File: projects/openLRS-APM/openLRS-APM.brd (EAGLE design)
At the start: 43.1 x 20.7 mm, 28 parts, among them IC1 MCP1703CB, IC2 RFM23BPSMD, J1 AVR_SPI_PRG_6PTH, U1 ATMEGA328P, Y1 16MHz

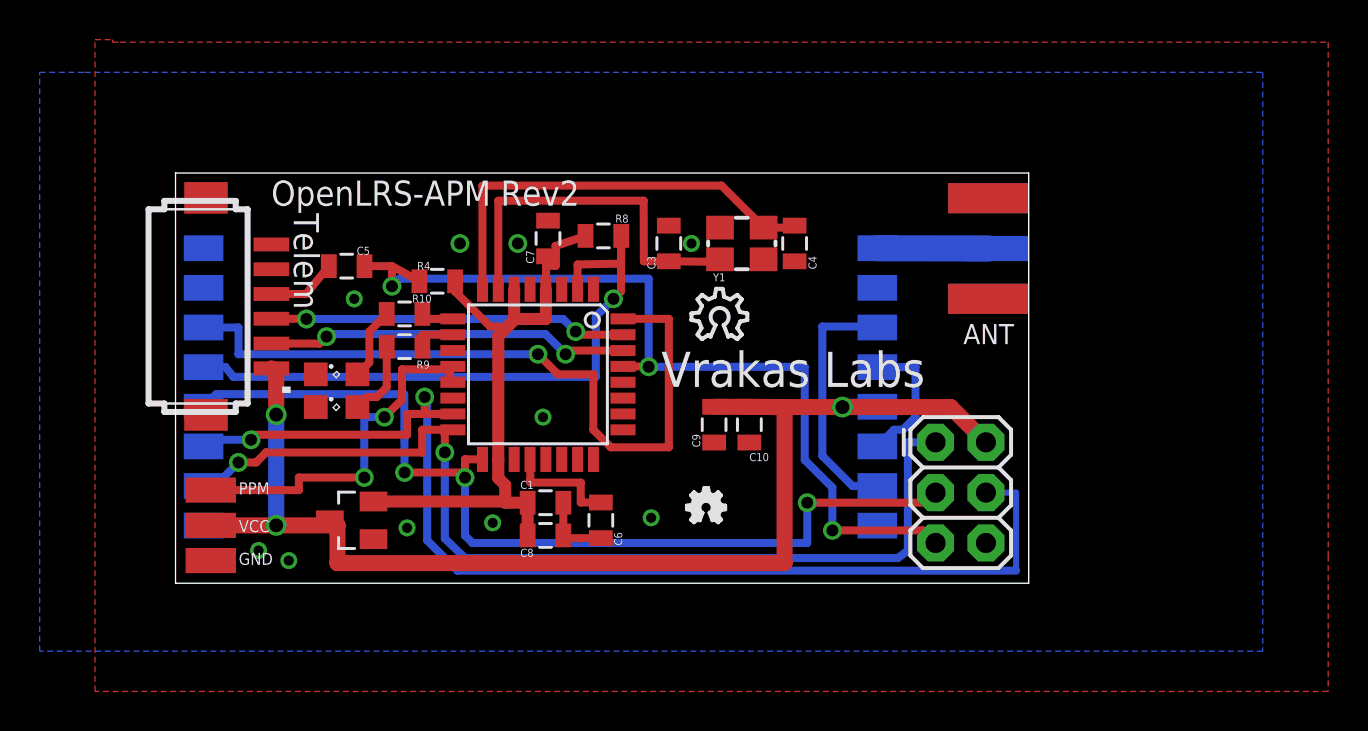
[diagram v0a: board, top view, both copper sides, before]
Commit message: Initial 32u4 USB dongle version
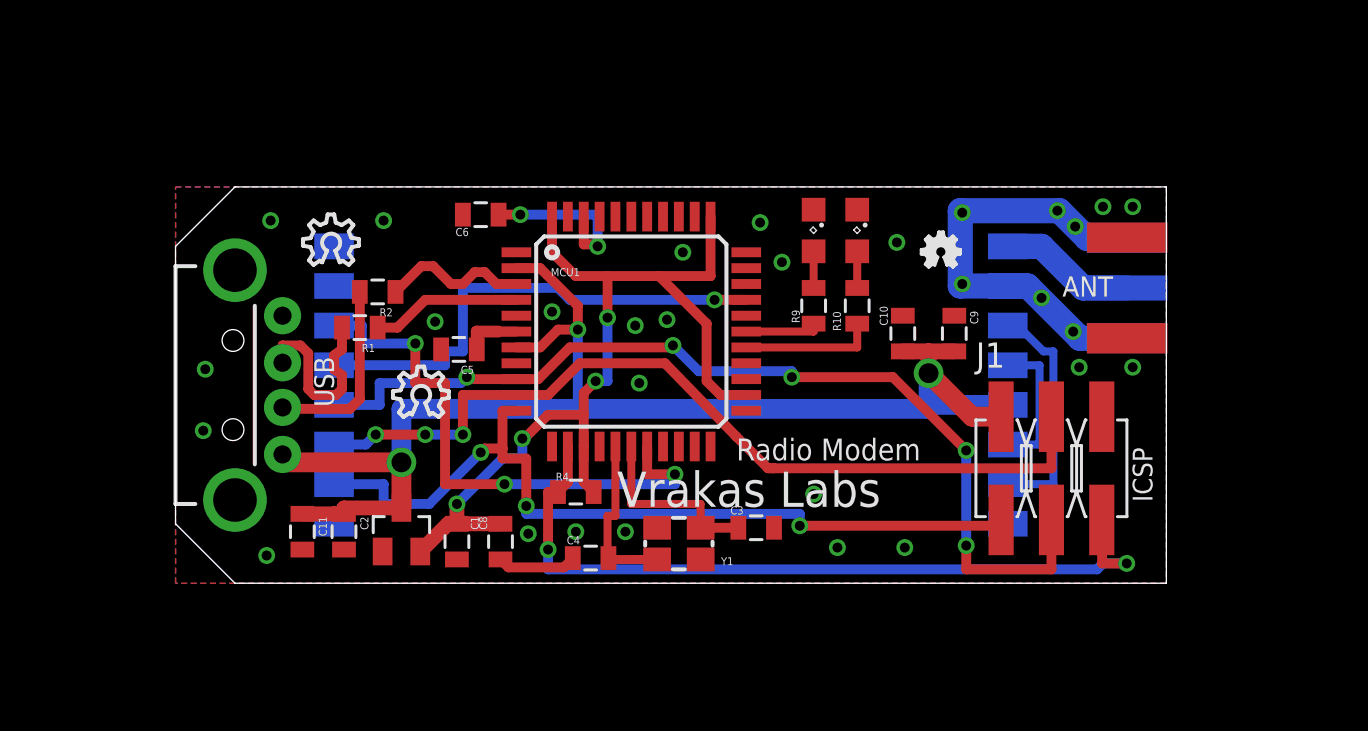
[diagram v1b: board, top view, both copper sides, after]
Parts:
- removed C7: 100n, SparkFun-Capacitors:0805
- removed GND, PPM, VCC: (no value), wirepad:SMD1,27-2,54
- removed R8: 1k, SparkFun-Resistors:0805
- removed TELEMETRY: DF13-6P-1.25H, con-hirose-df13:DF13A-6P-1.25H
- removed U1: ATMEGA328P, SparkFun-DigitalIC:TQFP32-08
- added C11: 100n, SparkFun-Capacitors:0805
- added C2: 1uF, SparkFun-Capacitors:0805
- added JP1: USB-A-H, SparkFun-Connectors:USB-A-H
- added MCU1: ATMEGA32U4TQFP, SparkFun-DigitalIC:SPARKFUN-DIGITALIC_TQFP44
- added R1, R2: 22, SparkFun-Resistors:0805
- C5: value 100n -> 1uF
- J1: value AVR_SPI_PRG_6PTH -> CON_HEADER_PRG_AVR_ICSP-SMD; device SparkFun-Connectors:2X3 -> dp_devices:M2X3_SMD
- moved U$3 31.7 mm to (11.0, 8.39), flipped to the top
- moved LED2 27.3 mm to (34.4, 17.8), turned to 270 degrees
- moved LED1 25.7 mm to (32.2, 17.8), turned to 270 degrees
- moved R10 22.8 mm to (34.4, 14.0), turned to 270 degrees
- moved R9 20.7 mm to (32.2, 14.0), turned to 270 degrees
- moved U$2 20.0 mm to (6.43, 16.1)
- moved C4 18.9 mm to (20.9, 1.27), turned to 180 degrees
- moved U$1 17.5 mm to (37.6, 15.9)
- moved C6 16.6 mm to (15.4, 18.6), turned to 0 degrees
- moved Y1 15.5 mm to (25.4, 2.00), turned to 0 degrees
- moved C3 15.0 mm to (29.3, 2.80), turned to 0 degrees
- moved C9 13.0 mm to (39.3, 12.6), turned to 90 degrees
- moved R4 12.7 mm to (20.2, 4.60)
- moved C10 9.01 mm to (36.7, 12.6), turned to 90 degrees
- moved SMA 7.28 mm to (50.1, 14.9)
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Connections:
- removed net DTR: C5.1, TELEMETRY.P$4
- removed net N$14: C6.2, U1.20
- removed net PPM: PPM.1, U1.12, U1.13
- removed net RF_CS: IC2.13, R8.1, U1.2
- removed net RF_IRQ: IC2.14, U1.32
- removed net RXD: TELEMETRY.P$2, U1.30
- removed net TXD: TELEMETRY.P$3, U1.31
- new net CS: IC2.13, MCU1.30
- new net D_N: MCU1.3, R2.1
- new net D_P: MCU1.4, R1.1
- new net IRQ: IC2.14, MCU1.18
- new net N$3: C6.2, MCU1.42
- new net R_N: JP1.D-, R2.2
- new net R_P: JP1.D+, R1.2
- new net UCAP: C5.1, MCU1.6
- net /RESET: now also MCU1.13; no longer C5.2, U1.29
- net 3V: now also MCU1.14, MCU1.24, MCU1.34, MCU1.44; no longer C7.1, R8.2, U1.18, U1.4, U1.6
- net 5V: now also C11.1, C2.1, JP1.VBUS, MCU1.2, MCU1.7; no longer TELEMETRY.P$1, VCC.1
- net GND: now also C11.2, C2.2, C5.2, JP1.GND, MCU1.15, MCU1.23, MCU1.35, MCU1.43, MCU1.5; no longer C7.2, GND.1, TELEMETRY.P$5, TELEMETRY.P$6, U1.21, U1.3, U1.5
- net MISO: now also MCU1.11; no longer U1.16
- net MOSI: now also MCU1.10; no longer U1.15
- net N$11: now also MCU1.17; no longer U1.7
- net N$12: now also MCU1.16; no longer U1.8
- net N$7: now also MCU1.28; no longer U1.10
- net N$8: now also MCU1.27; no longer U1.9
- net SCK: now also MCU1.9; no longer U1.17
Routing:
- net RF_IRQ: track 37.2 -> 0.00 mm, vias 1 -> 0
- net RF_CS: track 32.5 -> 0.00 mm, vias 1 -> 0
- net IRQ: track 0.00 -> 28.5 mm, vias 0 -> 3
- net CS: track 0.00 -> 24.9 mm, vias 0 -> 1
- net GND: track 3.70 -> 26.4 mm, vias 10 -> 30
- net PPM: track 18.6 -> 0.00 mm, vias 2 -> 0
- net RXD: track 18.4 -> 0.00 mm, vias 2 -> 0
- net TXD: track 18.1 -> 0.00 mm, vias 2 -> 0
- net 3V: track 32.5 -> 48.4 mm, vias 0 -> 4
- net MOSI: track 58.3 -> 43.9 mm, vias 2 -> 3
- net N$12: track 22.0 -> 11.1 mm
- net R_P: track 0.00 -> 9.59 mm
- net R_N: track 0.00 -> 9.58 mm
- net N$11: track 18.8 -> 9.49 mm
- net N$3: track 0.00 -> 8.80 mm, vias 0 -> 2
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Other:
- board size 43.1 x 20.7 mm -> 50 x 20 mm
- board text added: "ICSP"
- board text added: "Radio Modem"
- board text added: "USB"
- board text removed: "1"
- board text removed: "OpenLRS-APM Rev2"
- board text removed: "Telem"
